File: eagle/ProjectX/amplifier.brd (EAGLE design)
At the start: 88.6 x 54 mm, 37 parts, among them U1 TC4427COA, U10 TC4427COA, U11 TC4427COA, U12 TC4427COA, U17 TC4427COA, U18 TC4427COA, U19 TC4427COA, U2 TC4427COA, U20 TC4427COA, U25 TC4427COA, U26 TC4427COA, U27 TC4427COA, U28 TC4427COA, U5 TC4427COA, U6 TC4427COA, U9 TC4427COA

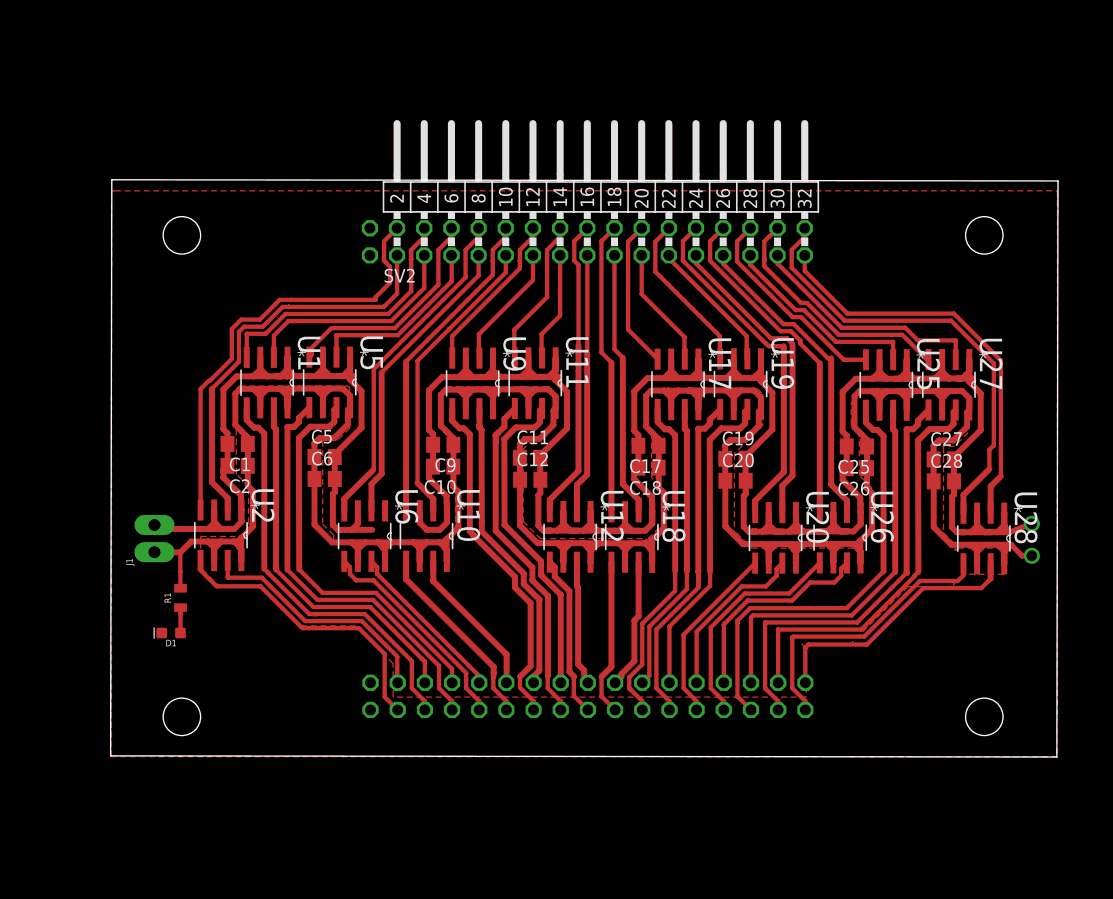
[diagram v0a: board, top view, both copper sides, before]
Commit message: changes
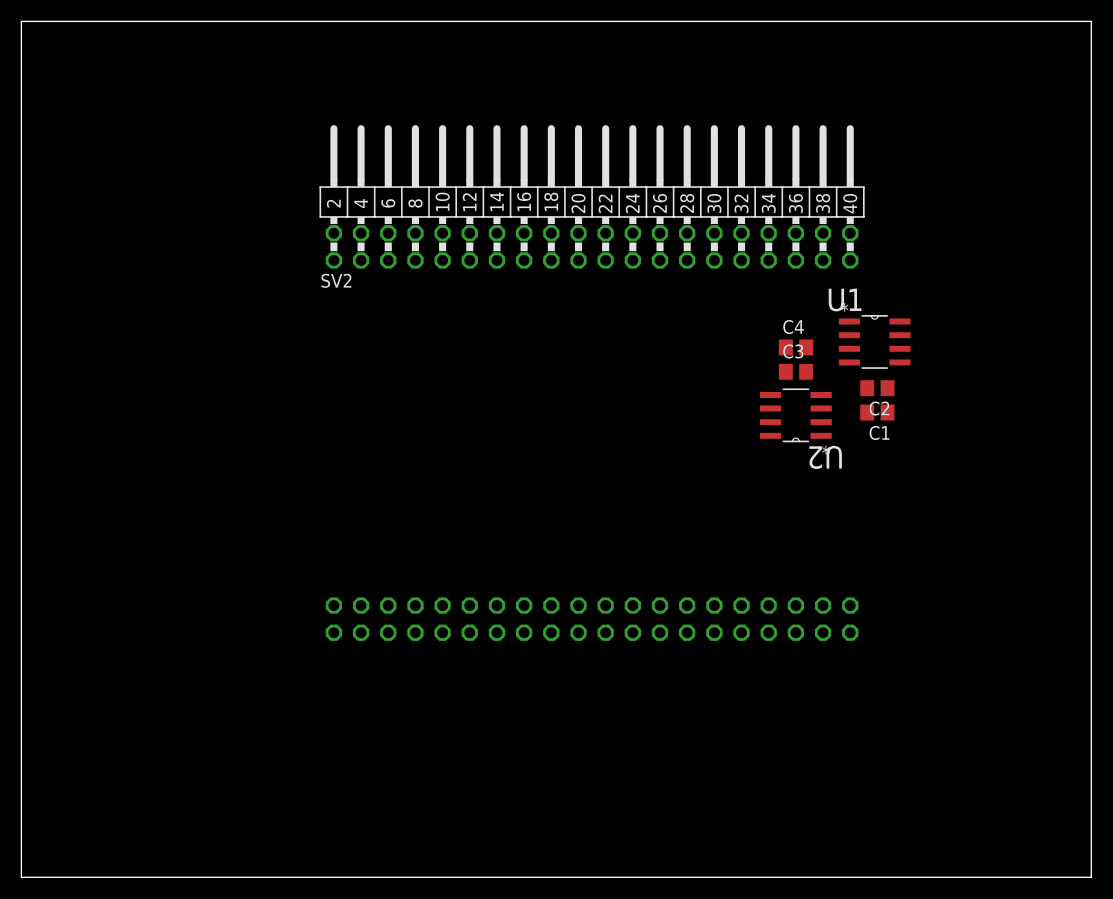
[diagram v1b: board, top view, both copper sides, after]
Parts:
- removed C10, C12, C18, C20, C26, C28, C6: 100nF, rcl:C0805
- removed C11, C17, C19, C25, C27, C5, C9: 4.7uF, rcl:C0805
- removed D1: (no value), SparkFun-LED:LED-0603
- removed J1: (no value), SparkFun-Connectors:1X02_LONGPADS
- removed R1: 1k, SparkFun-Resistors:0805
- removed U10, U11, U12, U17, U18, U19, U20, U25, U26, U27, U28, U5, U6, U9: TC4427COA, Microchip_By_element14_Batch_1:SOIC127P600X175-8N
- added C3: 4.7uF, rcl:C0805
- added C4: 100nF, rcl:C0805
- SV1, SV2: device Parts:MA20-2W -> con-lstb:MA20-2W
- moved C2 60.2 mm to (80.0, 45.7)
- moved C1 59.9 mm to (80.0, 43.4)
- moved U1 56.9 mm to (79.8, 50.0), turned to 0 degrees
- moved U2 54.9 mm to (72.4, 43.2), turned to 180 degrees
- moved SV1 9.36 mm to (53.3, 24.1)
- moved SV2 5.92 mm to (53.3, 58.9)
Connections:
- removed net N$10: SV1.1, U2.7
- removed net N$100: SV1.25, U26.7
- removed net N$101: SV1.26, U26.5
- removed net N$102: SV2.25, U26.2
- removed net N$103: SV1.27, U25.7
- removed net N$104: SV1.28, U25.5
- removed net N$105: SV2.30, U27.4
- removed net N$106: SV2.29, U27.2
- removed net N$107: SV2.32, U28.4
- removed net N$108: SV1.31, U28.7
- removed net N$109: SV1.32, U28.5
- removed net N$11: SV1.3, U1.7
- removed net N$110: SV2.31, U28.2
- removed net N$111: SV1.29, U27.7
- removed net N$112: SV1.30, U27.5
- removed net N$12: SV1.7, U6.7
- removed net N$13: SV1.10, U10.5
- removed net N$14: SV1.9, U10.7
- removed net N$15: SV1.11, U9.7
- removed net N$16: SV1.23, U20.7
- removed net N$17: SV2.6, U5.4
- removed net N$18: SV2.5, U5.2
- removed net N$19: SV2.8, U6.4
- removed net N$20: D1.A, R1.1
- removed net N$22: SV2.7, U6.2
- removed net N$23: SV1.5, U5.7
- removed net N$24: SV1.6, U5.5
- removed net N$26: SV1.15, U12.7
- removed net N$29: SV1.12, U9.5
- removed net N$33: SV2.12, U9.4
- removed net N$34: SV2.11, U9.2
- removed net N$35: SV2.10, U10.4
- removed net N$38: SV2.9, U10.2
- removed net N$41: SV2.14, U11.4
- removed net N$42: SV2.13, U11.2
- removed net N$43: SV2.16, U12.4
- removed net N$46: SV2.15, U12.2
- removed net N$47: SV1.13, U11.7
- removed net N$48: SV1.14, U11.5
- removed net N$65: SV2.20, U17.4
- removed net N$66: SV2.19, U17.2
- removed net N$67: SV2.18, U18.4
- removed net N$68: SV1.17, U18.7
- removed net N$69: SV1.18, U18.5
- removed net N$70: SV2.17, U18.2
- removed net N$71: SV1.19, U17.7
- removed net N$72: SV1.20, U17.5
- removed net N$73: SV2.22, U19.4
- removed net N$74: SV2.21, U19.2
- removed net N$75: SV2.24, U20.4
- removed net N$78: SV2.23, U20.2
- removed net N$79: SV1.21, U19.7
- removed net N$80: SV1.22, U19.5
- removed net N$9: SV1.8, U6.5
- removed net N$97: SV2.28, U25.4
- removed net N$98: SV2.27, U25.2
- removed net N$99: SV2.26, U26.4
- removed net VDD: C1.1, C10.1, C11.1, C12.1, C17.1, C18.1, C19.1, C2.1, C20.1, C25.1, C26.1, C27.1, C28.1, C5.1, C6.1, C9.1, J1.1, R1.2, U1.6, U1.8, U10.6, U10.8, U11.6, U11.8, U12.6, U12.8, U17.6, U17.8, U18.6, U18.8, U19.6, U19.8, U2.6, U2.8, U20.6, U20.8, U25.6, U25.8, U26.6, U26.8, U27.6, U27.8, U28.6, U28.8, U5.6, U5.8, U6.6, U6.8, U9.6, U9.8
- new net VCC: C1.1, C2.1, C3.1, C4.1, SV1.3, SV1.4, SV2.3, SV2.4, U1.6, U2.6
- net GND: now also C3.2, C4.2, SV1.1, SV1.2, SV2.1, SV2.2; no longer C10.2, C11.2, C12.2, C17.2, C18.2, C19.2, C20.2, C25.2, C26.2, C27.2, C28.2, C5.2, C6.2, C9.2, D1.C, J1.2, SV1.GND, SV1.GND+1, SV2.GND, SV2.GND+1, U1.1, U10.1, U10.3, U11.1, U11.3, U12.1, U12.3, U17.1, U17.3, U18.1, U18.3, U19.1, U19.3, U2.1, U20.1, U20.3, U25.1, U25.3, U26.1, U26.3, U27.1, U27.3, U28.1, U28.3, U5.1, U5.3, U6.1, U6.3, U9.1, U9.3
- net N$1: now also SV2.34; no longer SV2.2
- net N$2: now also SV1.39, U1.7; no longer SV1.2, U2.5
- net N$3: now also SV1.37; no longer SV1.4
- net N$4: now also SV2.38; no longer SV2.4
- net N$5: now also SV2.40; no longer SV2.3
- net N$6: now also SV2.36; no longer SV2.1
- net N$7: now also SV1.35, U2.7; no longer SV1.16, U12.5
- net N$8: now also SV1.33, U2.5; no longer SV1.24, U20.5
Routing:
- net VDD: track 334.7 -> 0.00 mm, vias 1 -> 0
- net GND: track 326.6 -> 0.00 mm, vias 1 -> 0
- net N$107: track 42.0 -> 0.00 mm
- net N$1: track 40.8 -> 0.00 mm
- net N$104: track 40.6 -> 0.00 mm
- net N$112: track 40.3 -> 0.00 mm
- net N$24: track 38.9 -> 0.00 mm
- net N$3: track 38.7 -> 0.00 mm
- net N$6: track 38.3 -> 0.00 mm
- net N$111: track 38.0 -> 0.00 mm
- net N$110: track 37.9 -> 0.00 mm
- net N$23: track 37.1 -> 0.00 mm
- net N$103: track 36.6 -> 0.00 mm
- net N$11: track 34.7 -> 0.00 mm
- net N$75: track 33.0 -> 0.00 mm
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- removed copper zone on layer 1, net GND
- removed copper zone on layer 1, net VDD
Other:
- board size 88.6 x 54 mm -> 100 x 80 mm
